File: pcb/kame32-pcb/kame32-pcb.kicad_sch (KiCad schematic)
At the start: 11 parts, among them J2 Conn_02x04_Odd_Even, J3 Conn_01x04, J4 Conn_01x04, J5 Conn_01x02, J6 Conn_02x04_Odd_Even, SW1 SW_SPDT, U1 TEA1-0505

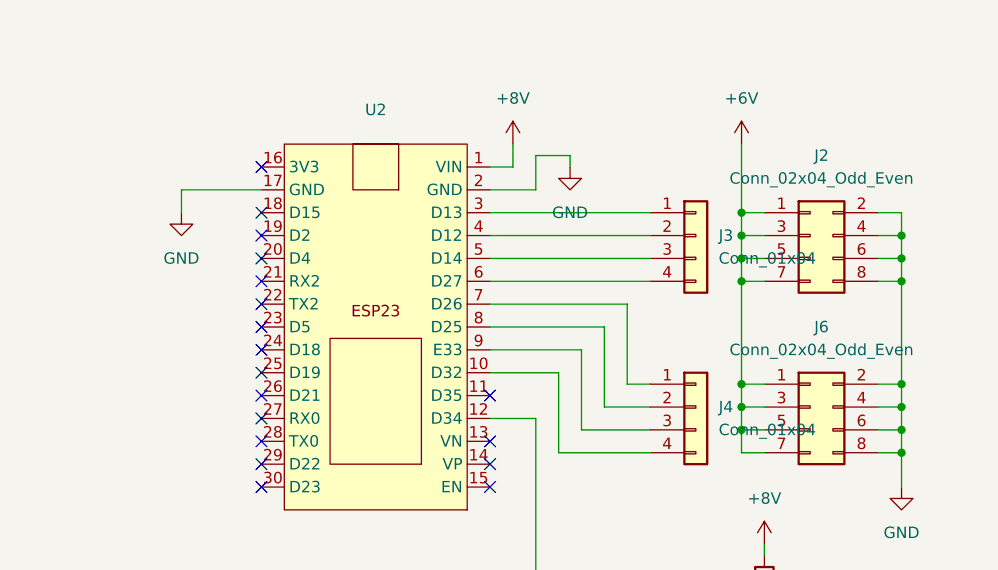
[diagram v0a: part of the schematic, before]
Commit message: PCB before DCDC change
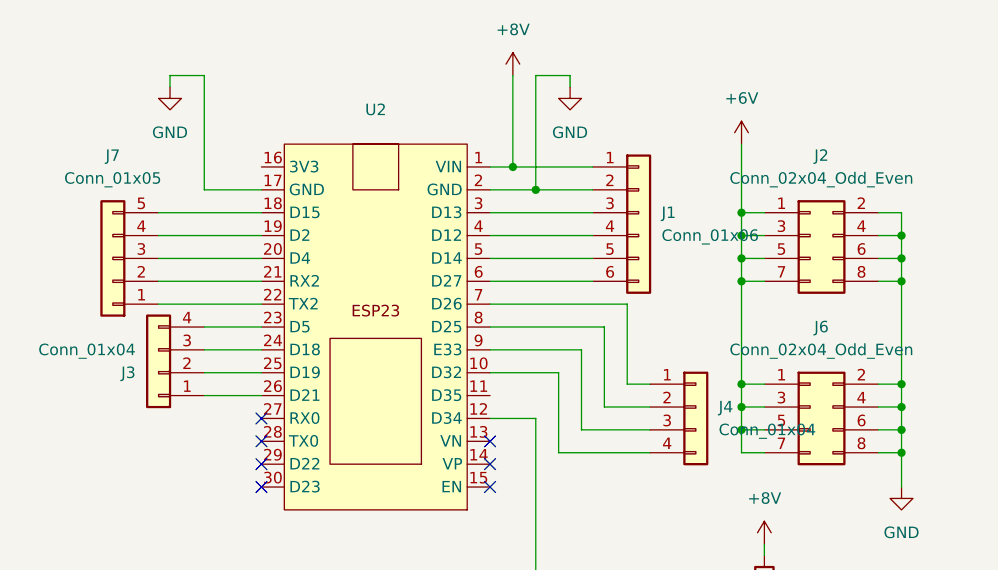
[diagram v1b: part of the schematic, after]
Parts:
- added J1: Conn_01x06, Connector_PinHeader_2.54mm:PinHeader_1x06_P2.54mm_Vertical, symbol Connector_Generic:Conn_01x06
- added J7: Conn_01x05, Connector_PinHeader_2.54mm:PinHeader_1x05_P2.54mm_Vertical, symbol Connector_Generic:Conn_01x05
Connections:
- net +8V: now also J1.1 (Pin_1)
- net -BATT: now also J1.2 (Pin_2)
- net at J3.1 (Pin_1): now also U2.26 (D21); no longer U2.3 (D13)
- net at J3.2 (Pin_2): now also U2.25 (D19); no longer U2.4 (D12)
- net at J3.3 (Pin_3): now also U2.24 (D18); no longer U2.5 (D14)
- net at J3.4 (Pin_4): now also U2.23 (D5); no longer U2.6 (D27)
- net at U2.18 (D15): now also J7.5 (Pin_5)
- net at U2.19 (D2): now also J7.4 (Pin_4)
- net at U2.20 (D4): now also J7.3 (Pin_3)
- net at U2.21 (RX2): now also J7.2 (Pin_2)
- net at U2.22 (TX2): now also J7.1 (Pin_1)
- new net: J1.3 (Pin_3), U2.3 (D13)
- new net: J1.4 (Pin_4), U2.4 (D12)
- new net: J1.5 (Pin_5), U2.5 (D14)
- new net: J1.6 (Pin_6), U2.6 (D27)
- no-connect marks 19 -> 8
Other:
- moved on the sheet: J3
